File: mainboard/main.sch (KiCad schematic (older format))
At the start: 1 part

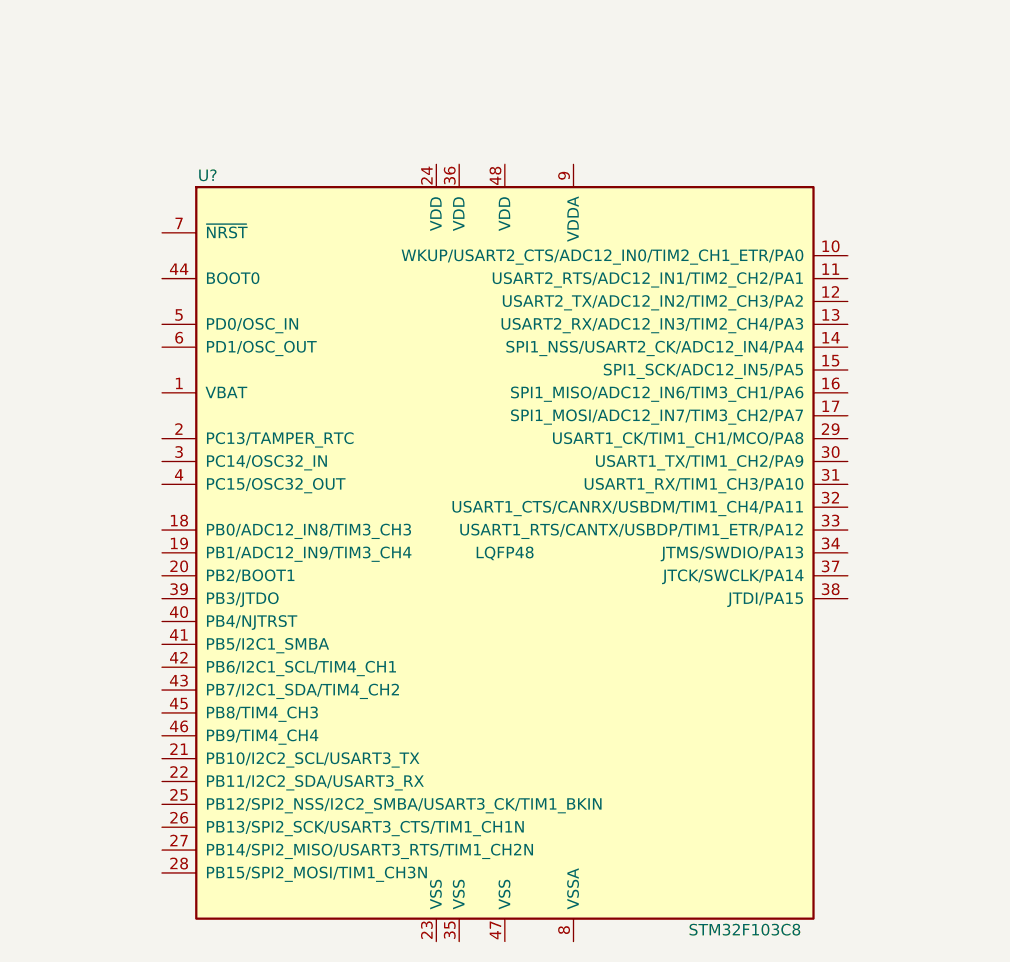
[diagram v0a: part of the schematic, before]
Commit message: nie chce misie
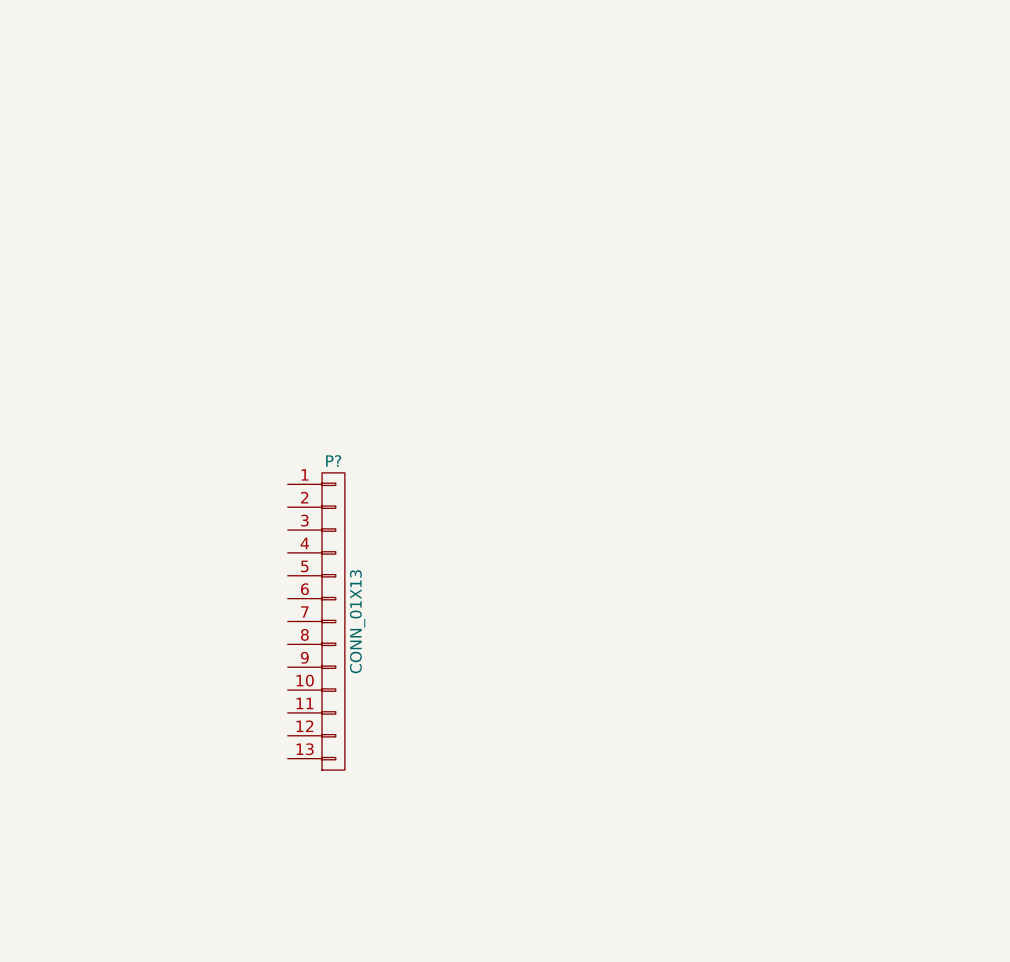
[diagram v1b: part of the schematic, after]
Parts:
- removed U?: STM32F103C8, LQFP48, symbol STM32F103C8
- added P?: CONN_01X13, symbol CONN_01X13
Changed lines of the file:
@@
 Comment4 ""
 $EndDescr
-$Comp
-L STM32F103C8 U?
-U 1 1 56C8F2D2
-P 6000 3450
-F 0 "U?" H 4700 5100 50  0000 C CNN
-F 1 "STM32F103C8" H 7050 1800 50  0000 C CNN
-F 2 "LQFP48" H 6000 3450 50  0000 C CNN
-F 3 "" H 6000 3450 50  0000 C CNN
-	1    6000 3450
-	1    0    0    -1
-$EndComp
 $Sheet
 S 750  700  1700 1750
@@
 F1 "dwm1000.sch" 60
 $EndSheet
+$Comp
+L CONN_01X13 P?
+U 1 1 56F99EBF
+P 5250 3750
+F 0 "P?" H 5250 4450 50  0000 C CNN
+F 1 "CONN_01X13" V 5350 3750 50  0000 C CNN
+F 2 "" H 5250 3750 50  0000 C CNN
+F 3 "" H 5250 3750 50  0000 C CNN
+	1    5250 3750
+	1    0    0    -1
+$EndComp
 $EndSCHEMATC
